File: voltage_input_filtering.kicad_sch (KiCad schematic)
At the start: 0 parts

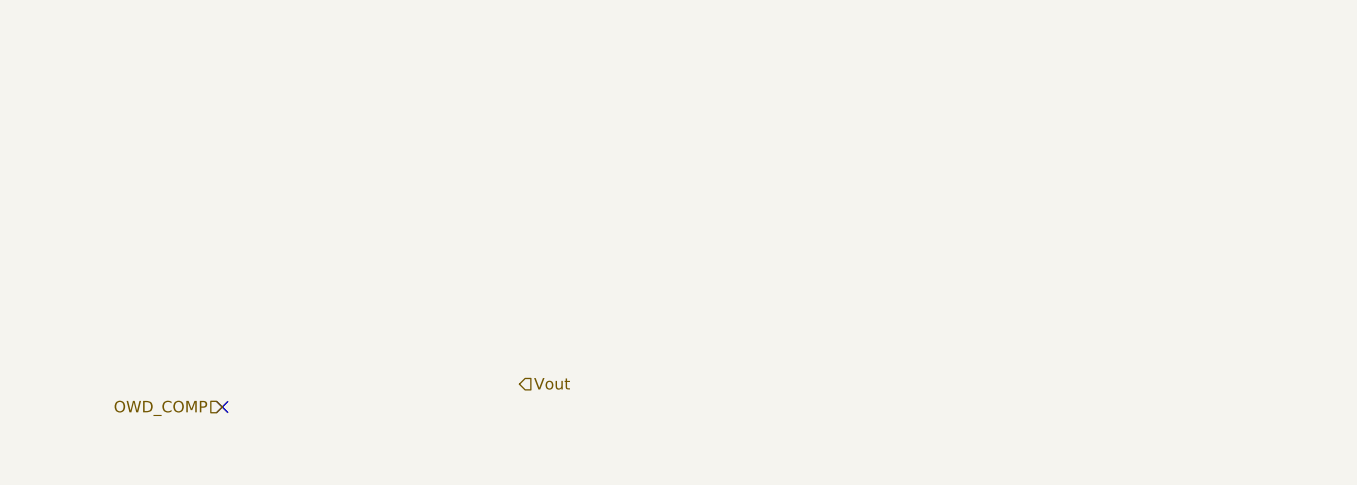
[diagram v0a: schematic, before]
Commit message: Launchpad controller revision 06/03/2024
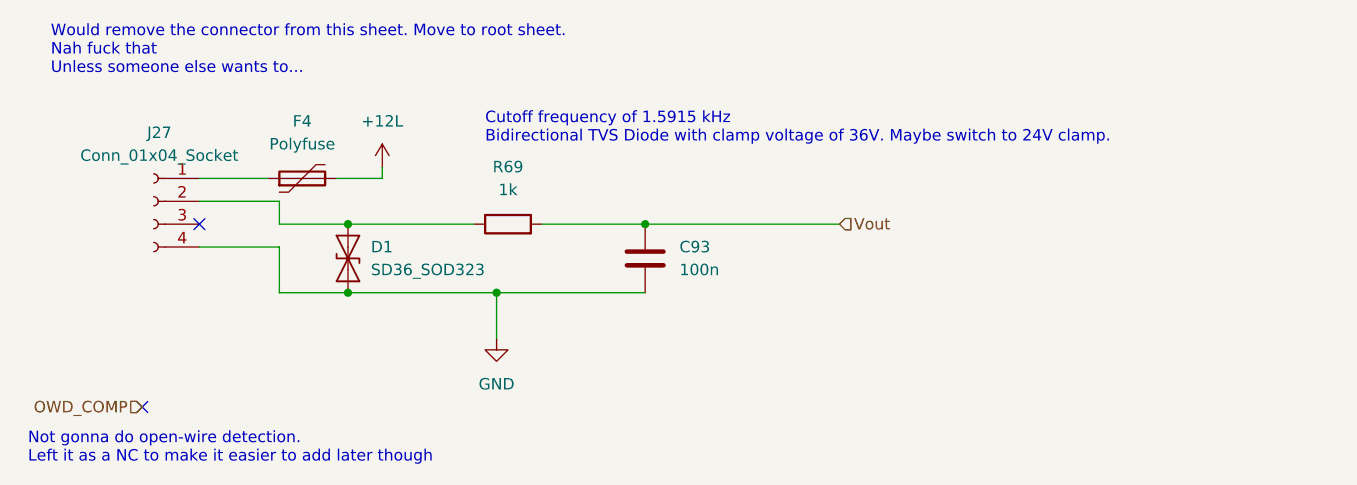
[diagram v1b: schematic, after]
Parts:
- added C93: 100n, symbol Device:C
- added D1: SD36_SOD323, Diode_SMD:D_SOD-323, symbol Diode:SD36_SOD323
- added F4: Polyfuse, symbol Device:Polyfuse
- added J27: Conn_01x04_Socket, symbol Connector:Conn_01x04_Socket
- added R69: 1k, symbol Device:R
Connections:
- net Vout: now also C93.1, R69.2
- new net: D1.2 (A2), J27.2 (Pin_2), R69.1
- new net: F4.1, J27.1 (Pin_1)
- new net +12L: F4.2
- new net GND: C93.2, D1.1 (A1), J27.4 (Pin_4)
- no-connect marks 1 -> 2
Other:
- note added: "Cutoff frequency of 1.5915 kHz Bidirectional TVS Diode with clamp voltage of 36V. Maybe switch to 24V clamp."
- note added: "Not gonna do open-wire detection. Left it as a NC to make it easier to add later though"
- note added: "Would remove the connector from this sheet. Move to root sheet. Nah fuck that Unless someone else wants to..."
